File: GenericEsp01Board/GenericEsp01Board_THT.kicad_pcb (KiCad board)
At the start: 2 copper layers, 43.8 x 21 mm, 13 parts, among them U1 ESP, U2 AMS1117

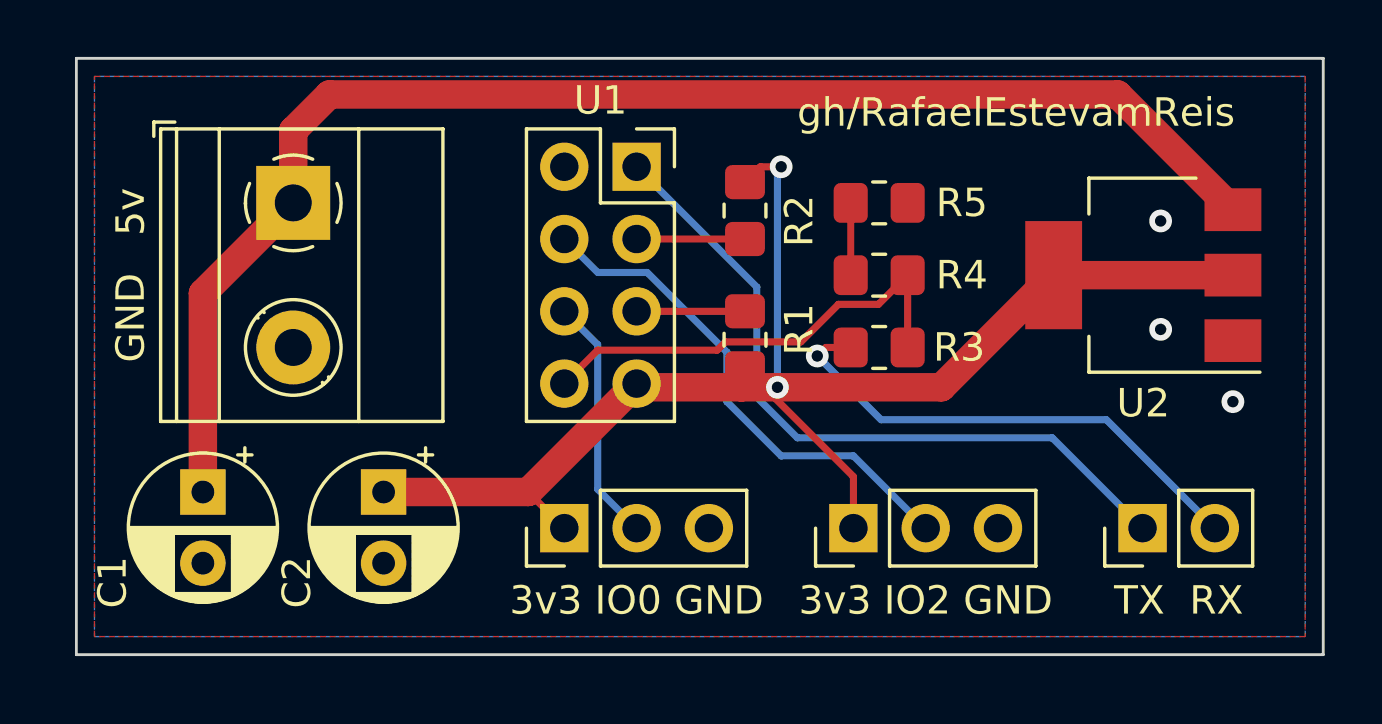
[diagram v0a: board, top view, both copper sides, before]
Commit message: Add THT
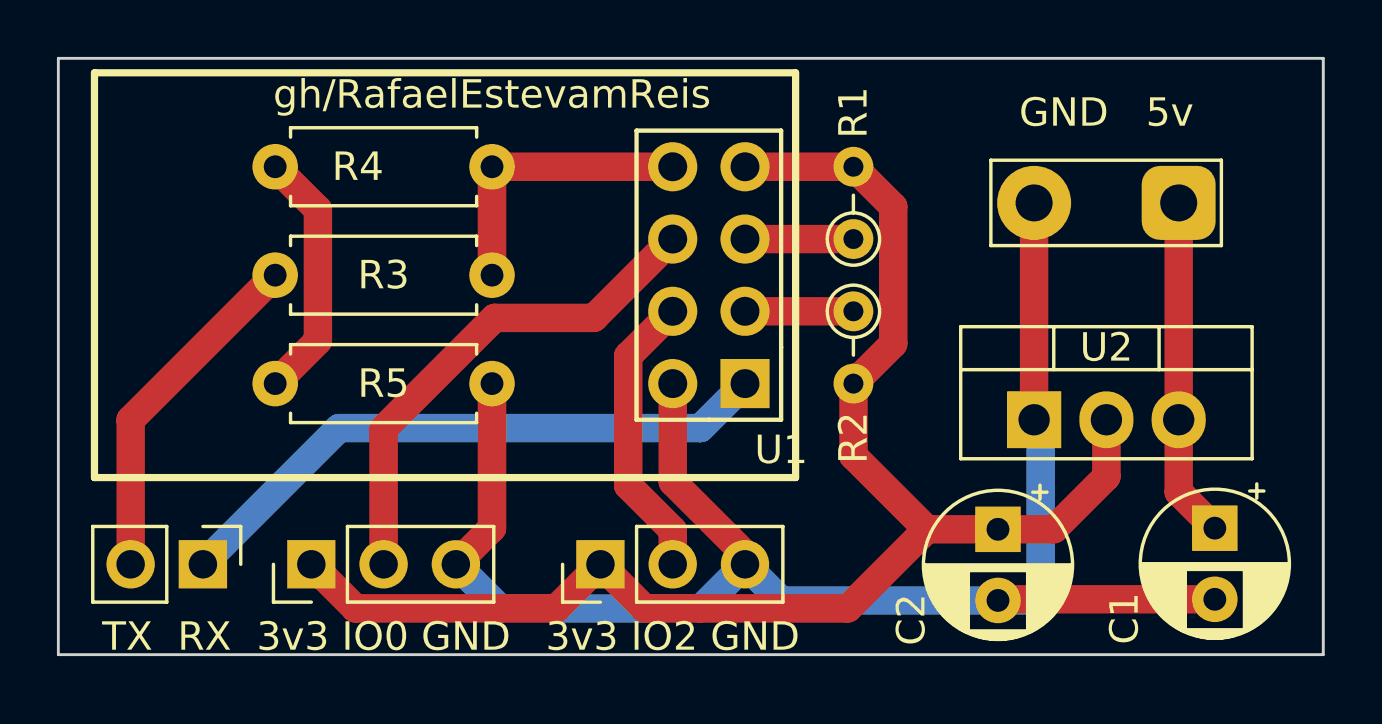
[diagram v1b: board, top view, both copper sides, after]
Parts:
- removed the GND   5v at (97.2, 105.4)
- added GND   5v: DC IN, TestPoint:TestPoint_2Pads_Pitch5.08mm_Drill1.3mm, F.Cu at (128.3, 105.4)
- R1, R2: footprint Resistor_SMD:R_0805_2012Metric_Pad1.20x1.40mm_HandSolder -> Resistor_THT:R_Axial_DIN0204_L3.6mm_D1.6mm_P2.54mm_Vertical
- R3, R4, R5: footprint Resistor_SMD:R_0805_2012Metric_Pad1.20x1.40mm_HandSolder -> Resistor_THT:R_Axial_DIN0207_L6.3mm_D2.5mm_P7.62mm_Horizontal
- U1: footprint Connector_PinSocket_2.54mm:PinSocket_2x04_P2.54mm_Vertical -> ESP:ESP-01
- U2: footprint Package_TO_SOT_SMD:SOT-223-3_TabPin2 -> Package_TO_SOT_THT:TO-220-3_Vertical
- moved C1 35.6 mm to (129.5, 116.8)
- moved TX  RX 33.0 mm to (94.0, 118.1), turned to 270 degrees
- moved C2 21.6 mm to (121.9, 116.9)
- moved R4 21.6 mm to (96.5, 104.1)
- moved R5 15.0 mm to (104.1, 111.8)
- moved R3 13.8 mm to (104.1, 108.0)
- moved 3v3 IO0 GND 8.98 mm to (97.8, 118.1)
- moved 3v3 IO2 GND 8.98 mm to (108.0, 118.1)
- moved U1 8.52 mm to (113.0, 111.8), turned to 180 degrees
- moved U2 6.37 mm to (123.2, 113.0), turned to 0 degrees
- moved R1 5.20 mm to (116.8, 106.7), turned to 90 degrees
- moved R2 5.20 mm to (116.8, 109.2), turned to 270 degrees
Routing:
- net GND: track 0.00 -> 58.1 mm, vias 3 -> 0
- net /DC_IN: track 49.2 -> 12.0 mm
- net /GPIO0: track 8.67 -> 17.7 mm
- net /GPIO2: track 17.9 -> 10.2 mm
- net Net-(R4-Pad1): track 2.54 -> 8.86 mm
- net /3v3_RX: track 16.2 -> 10.2 mm
- net Net-(J2-Pad2): track 17.8 -> 12.3 mm, vias 1 -> 0
- net /3v3_TX: track 25.3 -> 21.7 mm
- net /3v3: track 52.1 -> 52.6 mm, vias 2 -> 0
- removed copper zone on B.Cu, net GND
- removed copper zone on F.Cu, net GND
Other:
- board size 43.8 x 21 mm -> 44.4 x 21 mm
